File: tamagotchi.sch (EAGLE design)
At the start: 7 parts, among them U1 ATTINY84-20SSU

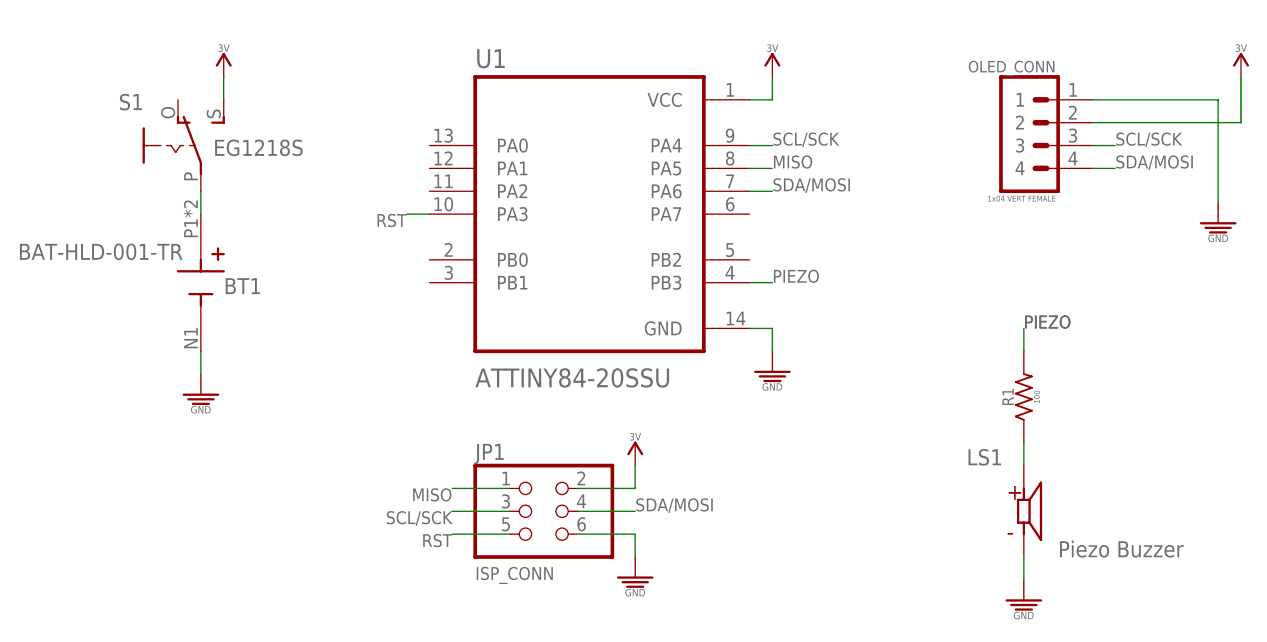
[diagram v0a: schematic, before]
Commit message: gerber
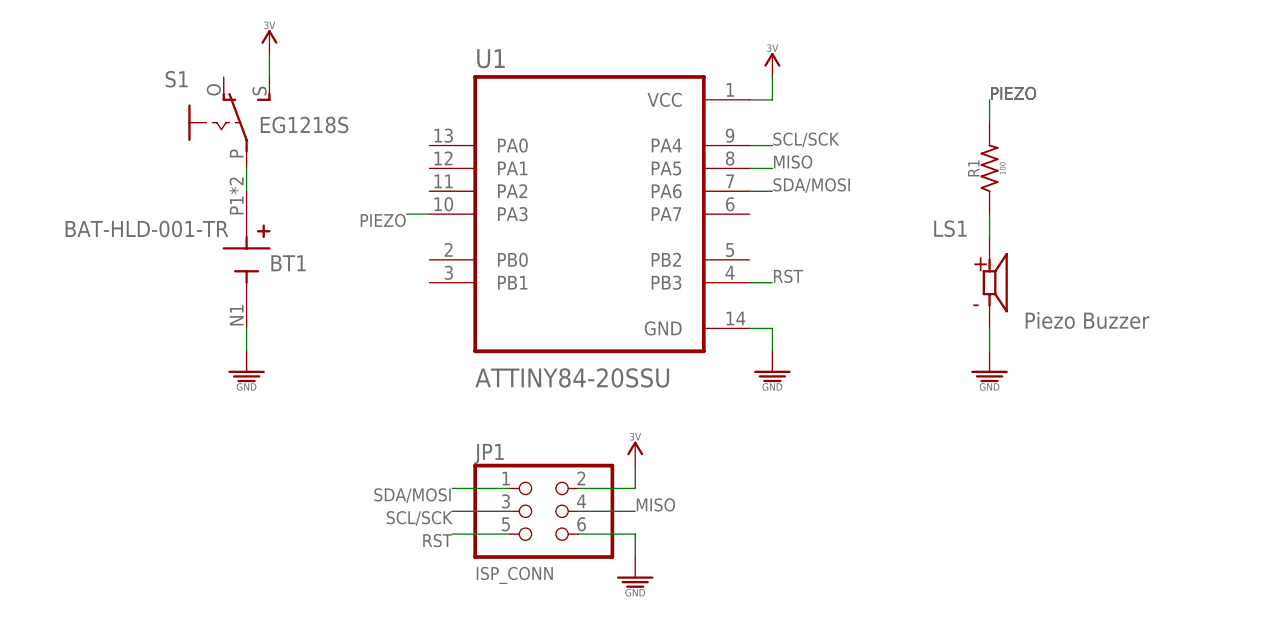
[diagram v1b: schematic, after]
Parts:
- removed OLED_CONN: 1x04 VERT FEMALE, PiB_connectors:1X04_PTH_VERT-FEMALE_2.54MM
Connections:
- net 3V: no longer OLED_CONN.2
- net GND: no longer OLED_CONN.1
- net MISO: now also JP1.4; no longer JP1.1
- net PIEZO: now also U1.PA3; no longer U1.PB3
- net RST: now also U1.PB3; no longer U1.PA3
- net SCL/SCK: no longer OLED_CONN.3
- net SDA/MOSI: now also JP1.1; no longer JP1.4, OLED_CONN.4
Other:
- moved on the sheet: BT1, LS1, R1, S1
